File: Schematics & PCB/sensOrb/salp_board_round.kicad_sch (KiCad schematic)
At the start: 77 parts, among them J1 Antenna, J10 COMM_SEL_0, J3 ATTINY3226, J4 POWER, J5 ATTINY3226, J7 READ/WRITE, J8 READ/WRITE, J9 COMM_SEL_1, Q1 IRLML6402, Q2 IRLML6402, U1 PN5321A3HN/C106_55, U2 ATtiny3226-S, U3 TP4057, U4 LD1117S33TR, U5 DW01A, Y1 27.12 MHz

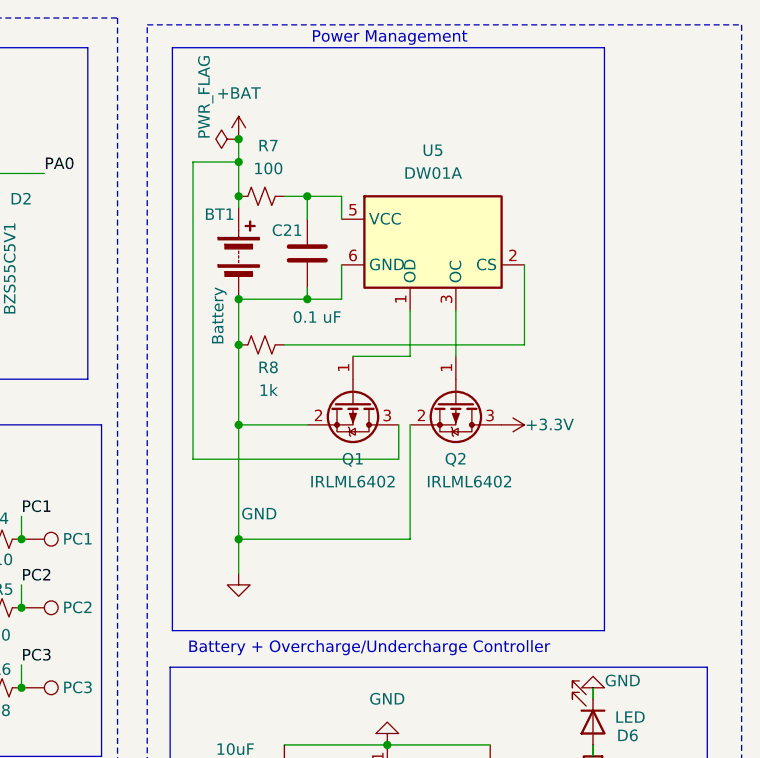
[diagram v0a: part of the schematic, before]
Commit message: Fixes To Battery Management
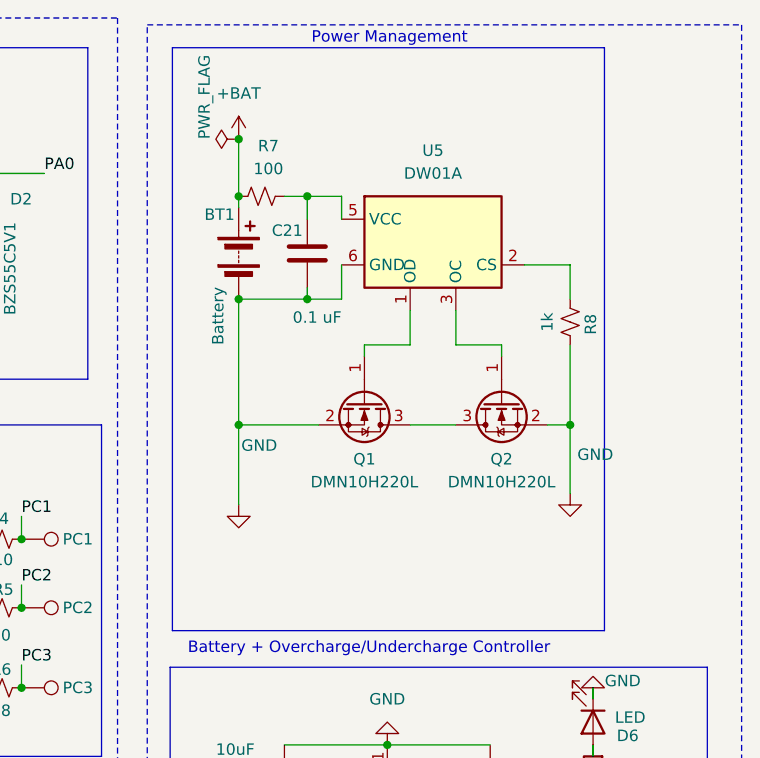
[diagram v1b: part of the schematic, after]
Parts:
- removed Q1, Q2: IRLML6402, Package_TO_SOT_SMD:SOT-23, symbol Transistor_FET:IRLML6402
- added Q1, Q2: DMN10H220L, Package_TO_SOT_SMD:SOT-23, symbol Transistor_FET:DMN10H220L
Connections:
- net GND: now also Q1.2 (S), Q2.2 (S)
- net at U5.1 (OD): now also Q1.1 (G)
- net at U5.3 (OC): now also Q2.1 (G)
- new net: Q1.3 (D), Q2.3 (D)
